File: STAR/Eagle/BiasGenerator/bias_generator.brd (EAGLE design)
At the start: 54.6 x 29.8 mm, 24 parts, among them J1 J30J-9J30, T1 750311838, U1 LT8300, U2 LT8330

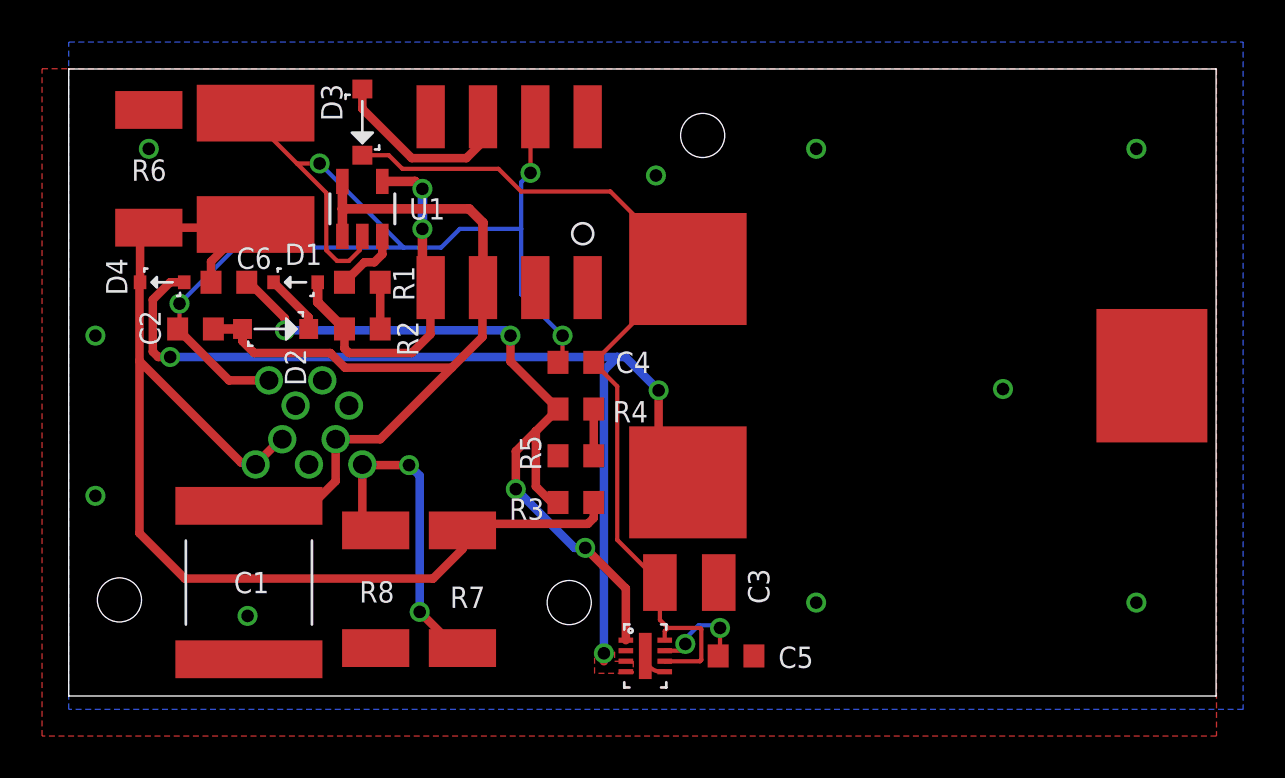
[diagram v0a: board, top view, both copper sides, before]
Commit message: misc board stuff
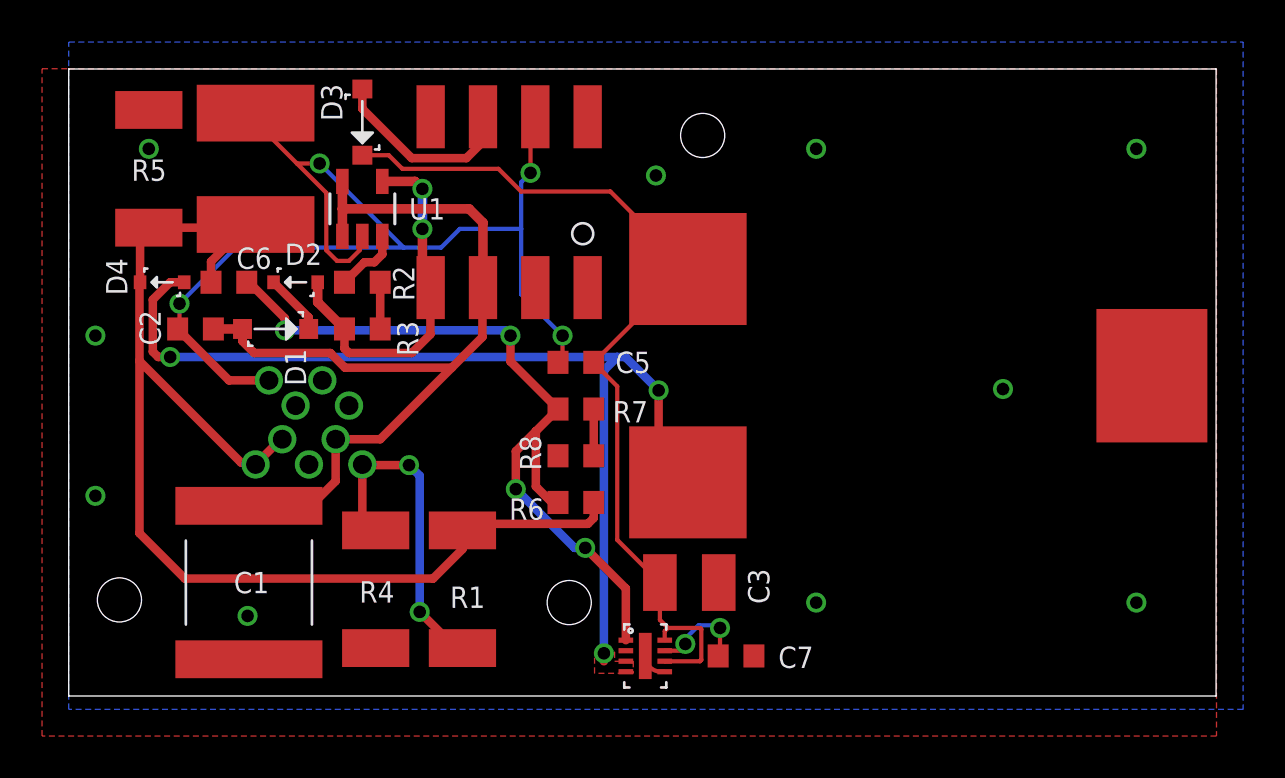
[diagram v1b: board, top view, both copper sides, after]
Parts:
- C4: value 1uF -> 10uF; device AR_passives:0603 -> AR_passives:2J-LEAD
- C7: value 10uF -> 1uF; device AR_passives:2J-LEAD -> AR_passives:0603
- D1: value BAV20W -> MMSZ5266BT1G; device AR_diode:SOD323 -> AR_diode:SOD123
- D2: value MMSZ5266BT1G -> BAV20W; device AR_diode:SOD123 -> AR_diode:SOD323
- R1: value 407k -> 47k; device resistor:R0603 -> resistor:R2512
- R2: value 1k -> 407k
- R3: value 1M -> 1k
- R4: value 1M -> 3k; device resistor:R0603 -> resistor:R2512
- R5: value 1M -> 1.5k; device resistor:R0603 -> resistor:R2512
- R6: value 1.5k -> 1M; device resistor:R2512 -> resistor:R0603
- R7: value 47k -> 1M; device resistor:R2512 -> resistor:R0603
- R8: value 3k -> 1M; device resistor:R2512 -> resistor:R0603
- moved C7 32.6 mm to (31.8, 2.54), turned to 0 degrees
- moved R6 25.8 mm to (24.1, 9.84), turned to 0 degrees
- moved R5 24.5 mm to (3.81, 25.7), turned to 270 degrees
- moved C4 17.8 mm to (8.89, 25.7), turned to 90 degrees
- moved C5 15.9 mm to (24.1, 16.5), turned to 180 degrees
- moved R1 15.4 mm to (18.7, 5.71), turned to 90 degrees
- moved R3 13.1 mm to (14.0, 18.1), turned to 180 degrees
- moved R4 12.8 mm to (14.6, 5.71), turned to 90 degrees
- moved R8 11.4 mm to (24.1, 12.1), turned to 0 degrees
- moved R7 10.1 mm to (24.1, 14.3), turned to 180 degrees
- moved D1 2.42 mm to (9.84, 18.1), turned to 0 degrees
- moved D2 2.42 mm to (10.8, 20.3), turned to 180 degrees
- moved R2 2.22 mm to (14.0, 20.3), turned to 0 degrees
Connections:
- net +20V: now also C5.1; no longer C4.1
- net +50V: now also C4.P$1, R1.2, R5.2; no longer C7.P$1, R3.2, R7.2
- net GND: now also C4.P$2, C7.2, R4.1; no longer C4.2, C7.P$2, R6.1
- net N$11: now also R7.1, R8.2; no longer R4.1, R5.2
- net N$2: now also R2.1; no longer R1.1
- net N$3: now also R2.2, R3.1; no longer R1.2, R2.1
- net N$4: now also D2.P$1, R3.2; no longer D1.P$1, R2.2
- net N$6: now also C7.1; no longer C5.1
- net N$9: now also R6.1, R7.2; no longer R3.1, R4.2
- net VCC: now also D1.P$1; no longer D2.P$1
- net V_DIVIDE: now also R1.1, R4.2; no longer R7.1, R8.2
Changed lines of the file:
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@@
 <attribute name="VALUE" x="27.6225" y="2.8575" size="1.27" layer="27"/>
 </element>
-<element name="C4" library="AR_passives" package="0603" value="1uF" x="24.13" y="16.51" smashed="yes" rot="R180">
+<element name="C5" library="AR_passives" package="0603" value="1uF" x="24.13" y="16.51" smashed="yes" rot="R180">
 <attribute name="NAME" x="27.686" y="17.018" size="1.016" layer="25" font="vector" rot="R180"/>
 <attribute name="VALUE" x="24.765" y="18.923" size="1.27" layer="27" rot="R180"/>
 </element>
-<element name="C5" library="AR_passives" package="0603" value="1uF" x="31.75" y="2.54" smashed="yes">
+<element name="C7" library="AR_passives" package="0603" value="1uF" x="31.75" y="2.54" smashed="yes">
 <attribute name="NAME" x="35.433" y="2.9845" size="1.016" layer="25" font="vector" rot="R180"/>
 <attribute name="VALUE" x="31.115" y="0.127" size="1.27" layer="27"/>
@@
 <attribute name="VALUE" x="6.985" y="17.907" size="1.27" layer="27"/>
 </element>
-<element name="C7" library="AR_passives" package="2J-LEAD" value="10uF" x="8.89" y="25.7175" smashed="yes" rot="R90">
+<element name="C4" library="AR_passives" package="2J-LEAD" value="10uF" x="8.89" y="25.7175" smashed="yes" rot="R90">
 <attribute name="NAME" x="5.89" y="23.7175" size="1.27" layer="27" rot="R90"/>
 <attribute name="VALUE" x="13.89" y="23.7175" size="1.27" layer="27" rot="R90"/>
 </element>
-<element name="D1" library="AR_diode" package="SOD323" value="BAV20W" x="10.795" y="20.32" smashed="yes" rot="R180">
+<element name="D2" library="AR_diode" package="SOD323" value="BAV20W" x="10.795" y="20.32" smashed="yes" rot="R180">
 <attribute name="NAME" x="10.2855" y="21.143" size="1.016" layer="25" font="vector"/>
 <attribute name="VALUE" x="11.595" y="21.77" size="0.6096" layer="27" rot="R180"/>
 </element>
-<element name="D2" library="AR_diode" package="SOD123" value="MMSZ5266BT1G" x="9.8425" y="18.0975" smashed="yes">
+<element name="D1" library="AR_diode" package="SOD123" value="MMSZ5266BT1G" x="9.8425" y="18.0975" smashed="yes">
 <attribute name="NAME" x="10.2805" y="17.1575" size="1.016" layer="25" font="vector" rot="R270"/>
 <attribute name="VALUE" x="8.2425" y="16.1975" size="0.8128" layer="27"/>
@@
 </element>
 <element name="L1" library="AR_passives" package="PQ2614" value="10uH" x="43.815" y="15.875" smashed="yes" rot="R270"/>
-<element name="R1" library="resistor" package="R0603" value="407k" x="13.97" y="20.32" smashed="yes">
+<element name="R2" library="resistor" package="R0603" value="407k" x="13.97" y="20.32" smashed="yes">
 <attribute name="NAME" x="16.4465" y="19.431" size="1.016" layer="25" font="vector" rot="R90"/>
 <attribute name="VALUE" x="13.335" y="18.415" size="1.27" layer="27"/>
 </element>
-<element name="R2" library="resistor" package="R0603" value="1k" x="13.97" y="18.0975" smashed="yes" rot="R180">
+<element name="R3" library="resistor" package="R0603" value="1k" x="13.97" y="18.0975" smashed="yes" rot="R180">
 <attribute name="NAME" x="15.621" y="18.4785" size="1.016" layer="25" font="vector" rot="R270"/>
 <attribute name="VALUE" x="14.605" y="20.0025" size="1.27" layer="27" rot="R180"/>
 </element>
-<element name="R3" library="resistor" package="R0603" value="1M" x="24.13" y="9.8425" smashed="yes">
+<element name="R6" library="resistor" package="R0603" value="1M" x="24.13" y="9.8425" smashed="yes">
 <attribute name="NAME" x="20.955" y="9.017" size="1.016" layer="25" font="vector"/>
 <attribute name="VALUE" x="23.495" y="7.9375" size="1.27" layer="27"/>
 </element>
-<element name="R4" library="resistor" package="R0603" value="1M" x="24.13" y="14.2875" smashed="yes" rot="R180">
+<element name="R7" library="resistor" package="R0603" value="1M" x="24.13" y="14.2875" smashed="yes" rot="R180">
 <attribute name="NAME" x="27.559" y="14.6685" size="1.016" layer="25" font="vector" rot="R180"/>
 <attribute name="VALUE" x="24.765" y="16.1925" size="1.27" layer="27" rot="R180"/>
 </element>
-<element name="R5" library="resistor" package="R0603" value="1M" x="24.13" y="12.065" smashed="yes">
+<element name="R8" library="resistor" package="R0603" value="1M" x="24.13" y="12.065" smashed="yes">
 <attribute name="NAME" x="22.479" y="11.3665" size="1.016" layer="25" font="vector" rot="R90"/>
 <attribute name="VALUE" x="23.495" y="10.16" size="1.27" layer="27"/>
 </element>
-<element name="R6" library="resistor" package="R2512" value="1.5k" x="3.81" y="25.7175" smashed="yes" rot="R270">
+<element name="R5" library="resistor" package="R2512" value="1.5k" x="3.81" y="25.7175" smashed="yes" rot="R270">
 <attribute name="NAME" x="2.9845" y="25.146" size="1.016" layer="25" font="vector"/>
 <attribute name="VALUE" x="0.635" y="28.2575" size="1.27" layer="27" rot="R270"/>
@@
 </element>
 <element name="U2" library="AR_IC" package="8-DFN" value="LT8330" x="27.432" y="2.54" smashed="yes" rot="R270"/>
-<element name="R7" library="resistor" package="R2512" value="47k" x="18.7325" y="5.715" smashed="yes" rot="R90">
+<element name="R1" library="resistor" package="R2512" value="47k" x="18.7325" y="5.715" smashed="yes" rot="R90">
 <attribute name="NAME" x="19.812" y="5.842" size="1.016" layer="25" font="vector" rot="R180"/>
 <attribute name="VALUE" x="21.9075" y="3.175" size="1.27" layer="27" rot="R90"/>
 </element>
-<element name="R8" library="resistor" package="R2512" value="3k" x="14.605" y="5.715" smashed="yes" rot="R90">
+<element name="R4" library="resistor" package="R2512" value="3k" x="14.605" y="5.715" smashed="yes" rot="R90">
 <attribute name="NAME" x="15.494" y="6.096" size="1.016" layer="25" font="vector" rot="R180"/>
 <attribute name="VALUE" x="17.78" y="3.175" size="1.27" layer="27" rot="R90"/>
@@
 <contactref element="U1" pad="5"/>
 <contactref element="C2" pad="1"/>
-<contactref element="D2" pad="P$1"/>
+<contactref element="D1" pad="P$1"/>
 <contactref element="T1" pad="P$3"/>
 <contactref element="C1" pad="P$1"/>
@@
 <contactref element="T1" pad="P$7"/>
 <contactref element="C3" pad="2"/>
-<contactref element="C4" pad="2"/>
 <contactref element="C5" pad="2"/>
+<contactref element="C7" pad="2"/>
 <contactref element="U2" pad="P$5"/>
 <contactref element="U2" pad="P$9"/>
+<contactref element="R8" pad="1"/>
+<contactref element="C4" pad="P$2"/>
 <contactref element="R5" pad="1"/>
-<contactref element="C7" pad="P$2"/>
-<contactref element="R6" pad="1"/>
-<contactref element="R8" pad="1"/>
+<contactref element="R4" pad="1"/>
 <contactref element="J1" pad="7"/>
 <polygon width="0.4064" layer="1" rank="6">
@@
 </signal>
 <signal name="N$1">
+<contactref element="D1" pad="P$2"/>
 <contactref element="D2" pad="P$2"/>
-<contactref element="D1" pad="P$2"/>
 <wire x1="11.4175" y1="18.0975" x2="11.4175" y2="18.6475" width="0.4064" layer="1"/>
 <wire x1="11.4175" y1="18.6475" x2="9.745" y2="20.32" width="0.4064" layer="1"/>
@@
 <signal name="N$4">
 <contactref element="U1" pad="4"/>
-<contactref element="D1" pad="P$1"/>
-<contactref element="R2" pad="2"/>
+<contactref element="D2" pad="P$1"/>
+<contactref element="R3" pad="2"/>
 <contactref element="T1" pad="P$4"/>
 <wire x1="11.845" y1="20.32" x2="11.845" y2="19.3725" width="0.4572" layer="1"/>
@@
 <contactref element="D3" pad="P$2"/>
 <contactref element="C3" pad="1"/>
-<contactref element="C4" pad="1"/>
+<contactref element="C5" pad="1"/>
 <contactref element="L1" pad="P$2"/>
 <contactref element="U2" pad="P$6"/>
@@
 </signal>
 <signal name="N$6">
-<contactref element="C5" pad="1"/>
+<contactref element="C7" pad="1"/>
 <contactref element="U2" pad="P$7"/>
 <wire x1="28.357" y1="2.79" x2="29.2695" y2="2.79" width="0.2032" layer="1"/>
@@
 <contactref element="U2" pad="P$1"/>
 <contactref element="C6" pad="2"/>
-<contactref element="R3" pad="1"/>
-<contactref element="R4" pad="2"/>
+<contactref element="R6" pad="1"/>
+<contactref element="R7" pad="2"/>
 <via x="10.287" y="18.034" extent="1-16" drill="0.6"/>
 <wire x1="10.287" y1="18.034" x2="20.7645" y2="18.034" width="0.4064" layer="16"/>
@@
 <signal name="N$2">
 <contactref element="U1" pad="3"/>
-<contactref element="R1" pad="1"/>
+<contactref element="R2" pad="1"/>
 <wire x1="14.5415" y1="21.2725" x2="14.92" y2="21.651" width="0.4064" layer="1"/>
 <wire x1="14.92" y1="21.651" x2="14.92" y2="22.5065" width="0.4064" layer="1"/>
@@
 </signal>
 <signal name="N$3">
-<contactref element="R2" pad="1"/>
-<contactref element="R1" pad="2"/>
+<contactref element="R3" pad="1"/>
+<contactref element="R2" pad="2"/>
 <wire x1="14.82" y1="18.0975" x2="14.82" y2="20.32" width="0.4064" layer="1"/>
 </signal>
 <signal name="+50V">
 <contactref element="C6" pad="1"/>
-<contactref element="R3" pad="2"/>
+<contactref element="R6" pad="2"/>
 <contactref element="D4" pad="P$2"/>
-<contactref element="C7" pad="P$1"/>
-<contactref element="R6" pad="2"/>
-<contactref element="R7" pad="2"/>
+<contactref element="C4" pad="P$1"/>
+<contactref element="R5" pad="2"/>
+<contactref element="R1" pad="2"/>
 <wire x1="3.81" y1="22.9175" x2="8.382" y2="22.9175" width="0.4064" layer="1"/>
 <wire x1="8.382" y1="22.9175" x2="8.74" y2="22.9175" width="0.4064" layer="1"/>
@@
 </signal>
 <signal name="N$11">
-<contactref element="R4" pad="1"/>
-<contactref element="R5" pad="2"/>
+<contactref element="R7" pad="1"/>
+<contactref element="R8" pad="2"/>
 <wire x1="24.98" y1="14.2875" x2="24.98" y2="12.065" width="0.4064" layer="1"/>
 </signal>
 <signal name="V_DIVIDE">
 <contactref element="J1" pad="5"/>
-<contactref element="R7" pad="1"/>
-<contactref element="R8" pad="2"/>
+<contactref element="R1" pad="1"/>
+<contactref element="R4" pad="2"/>
 <wire x1="18.7325" y1="2.915" x2="18.421" y2="2.915" width="0.4064" layer="1"/>
 <wire x1="18.421" y1="2.915" x2="16.7005" y2="4.6355" width="0.4064" layer="1"/>
